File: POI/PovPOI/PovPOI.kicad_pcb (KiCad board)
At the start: 2 copper layers, 21.7 x 46 mm, 19 parts, among them J1 Conn_02x08_Top_Bottom, J2 Conn_02x08_Top_Bottom, J3 Conn_01x04, J5 Conn_01x04

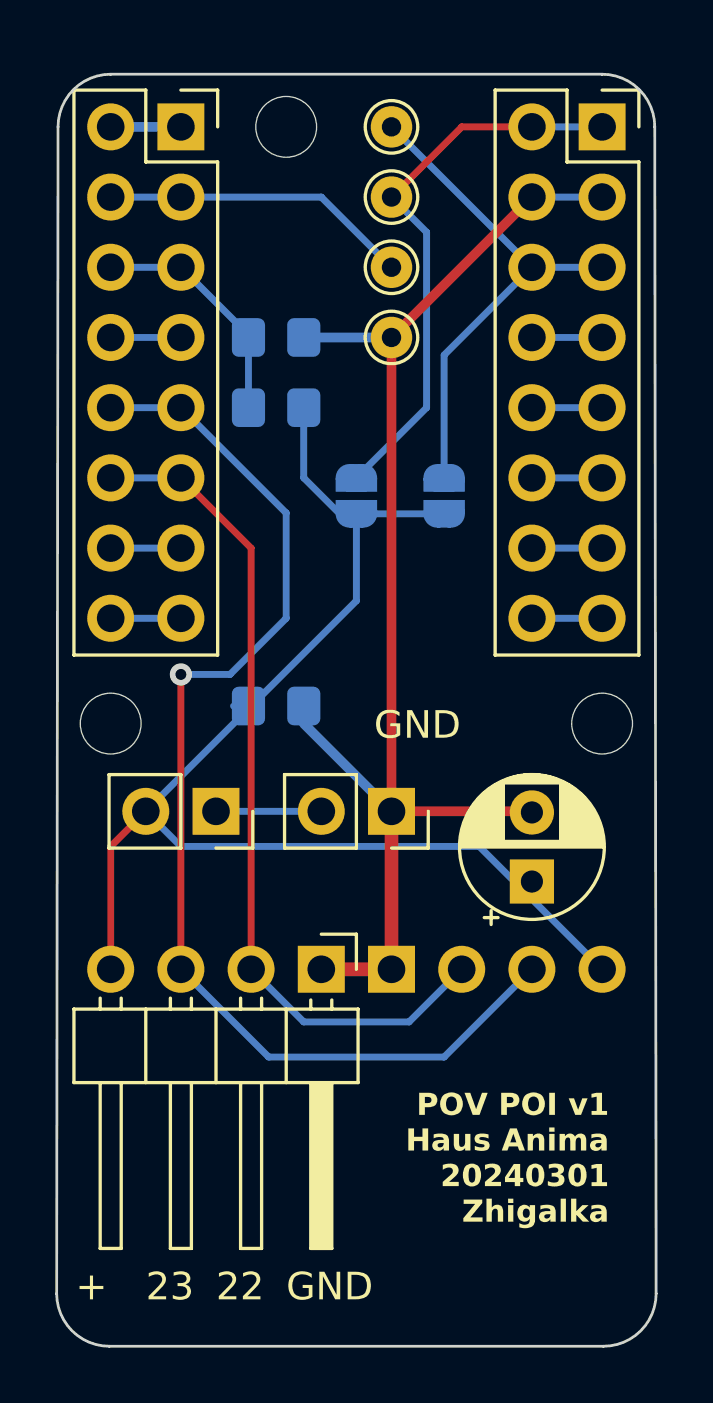
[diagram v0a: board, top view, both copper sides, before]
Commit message: POV POI v2, working towards v3
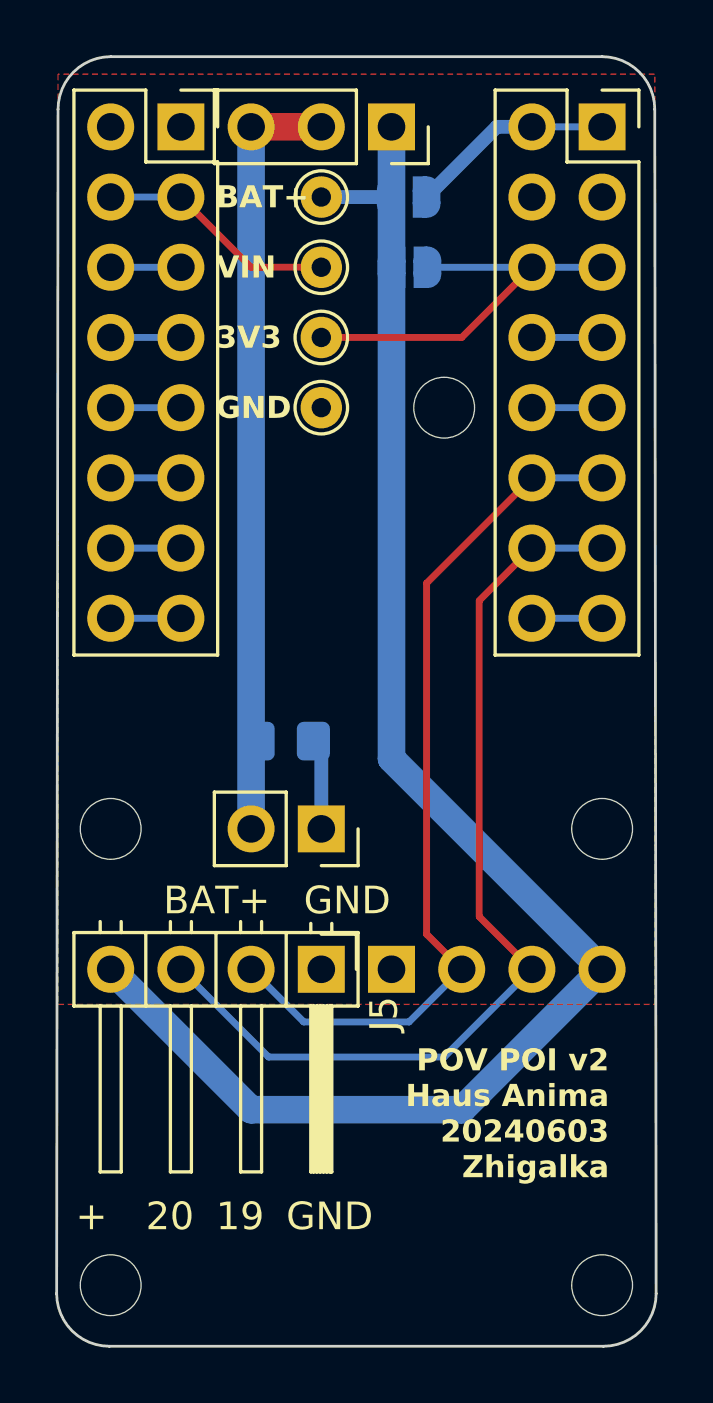
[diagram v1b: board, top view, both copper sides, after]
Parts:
- removed BatteryOnSW1: SW_SPST, Connector_PinSocket_2.54mm:PinSocket_1x02_P2.54mm_Vertical
- removed C1: C_Polarized, Capacitor_THT:CP_Radial_D5.0mm_P2.50mm
- removed R1, R2: R_Small, Resistor_SMD:R_0805_2012Metric_Pad1.20x1.40mm_HandSolder
- added H4: MountingHole, MountingHole:MountingHole_2.2mm_M2, F.Cu at (45.7, 69.8)
- added H5: MountingHole, MountingHole:MountingHole_2.2mm_M2, F.Cu at (40.0, 38.1)
- added SW1: SW_SPDT, Connector_PinSocket_2.54mm:PinSocket_1x03_P2.54mm_Vertical, F.Cu at (38.1, 27.9)
- J3, J5: footprint Connector_PinHeader_2.54mm:PinHeader_1x04_P2.54mm_Horizontal -> Library:PinHeader_1x04_P2.54mm_Horizontal_Seth
- moved H1 27.9 mm to (45.7, 53.3)
- moved H3 27.0 mm to (27.9, 69.8)
- moved JP1 11.0 mm to (38.7, 30.5), turned to 0 degrees
- moved JP2 8.36 mm to (38.8, 33.0), turned to 0 degrees
- moved TP3 8.03 mm to (35.6, 35.6)
- moved H2 3.81 mm to (27.9, 53.3)
- moved TP4 3.59 mm to (35.6, 38.1)
- moved BatteryConn1 2.62 mm to (35.6, 53.3)
- moved TP1 2.54 mm to (35.6, 30.5)
- moved TP2 2.54 mm to (35.6, 33.0)
- moved C2 1.32 mm to (34.3, 50.2)
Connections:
- C2 pad 1: /PCB_BAT -> /BAT_TERMINAL
- J3 pad 2: /22 -> /19
- J3 pad 3: /23 -> /20
- J3 pad 4: /PCB_BAT -> /PCB_BAT_ON
- J5 pad 2: /22 -> /19
- J5 pad 3: /23 -> /20
- J5 pad 4: /PCB_BAT -> /PCB_BAT_ON
- JP1 pad 1: /PCB_BAT -> /PCB_BAT_ON
- JP2 pad 1: /PCB_BAT -> /PCB_BAT_ON
- TP1 pad 1: /CHIP_BAT+ -> /PCB_BAT_ON
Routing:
- net /PCB_BAT_ON: track 0.00 -> 58.2 mm
- net /PCB_BAT: track 48.4 -> 0.00 mm
- net GND: track 50.7 -> 3.29 mm
- net /23: track 42.4 -> 2.54 mm, vias 1 -> 0
- net /20: track 2.54 -> 34.7 mm
- net /19: track 2.54 -> 31.6 mm
- net /22: track 30.6 -> 2.54 mm
- net /BAT_TERMINAL: track 3.81 -> 27.9 mm
- net /CHIP_BAT+: track 20.4 -> 7.40 mm
- net /4: track 8.63 -> 2.54 mm
- net /VIN: track 18.7 -> 15.0 mm
- net /3V3: track 11.2 -> 8.67 mm
- added copper zone on F.Cu, net GND
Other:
- board size 21.7 x 46 mm -> 21.7 x 46.7 mm
- board text added: "19"
- board text added: "20"
- board text added: "3V3"
- board text added: "BAT+"
- board text added: "POV POI v2 Haus Anima 20240603 Zhigalka"
- board text added: "VIN"
- board text removed: "22"
- board text removed: "23"
- board text removed: "POV POI v1 Haus Anima 20240301 Zhigalka"
